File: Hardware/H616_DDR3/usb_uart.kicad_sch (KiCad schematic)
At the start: 5 parts, among them J3 USB_C_Receptacle_USB2.0

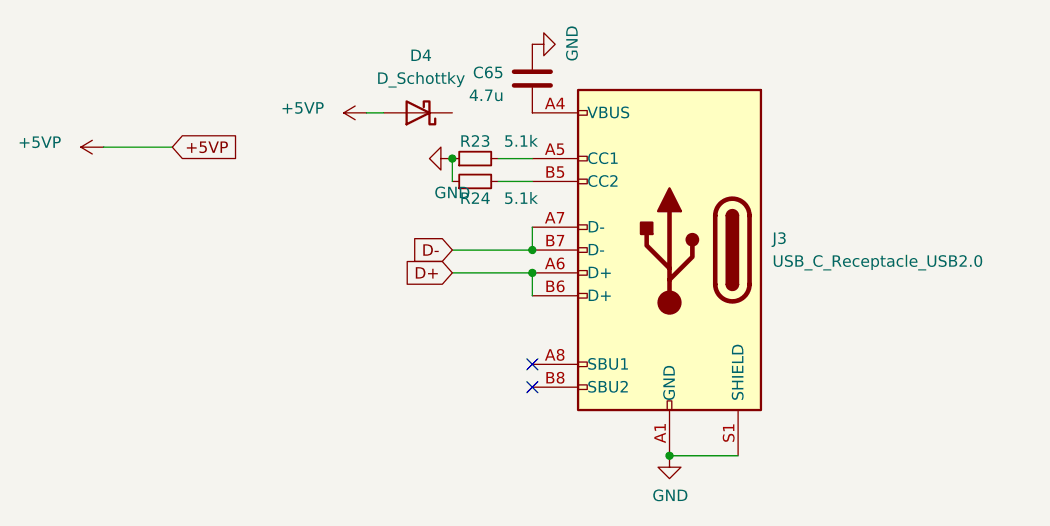
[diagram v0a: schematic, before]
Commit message: trace
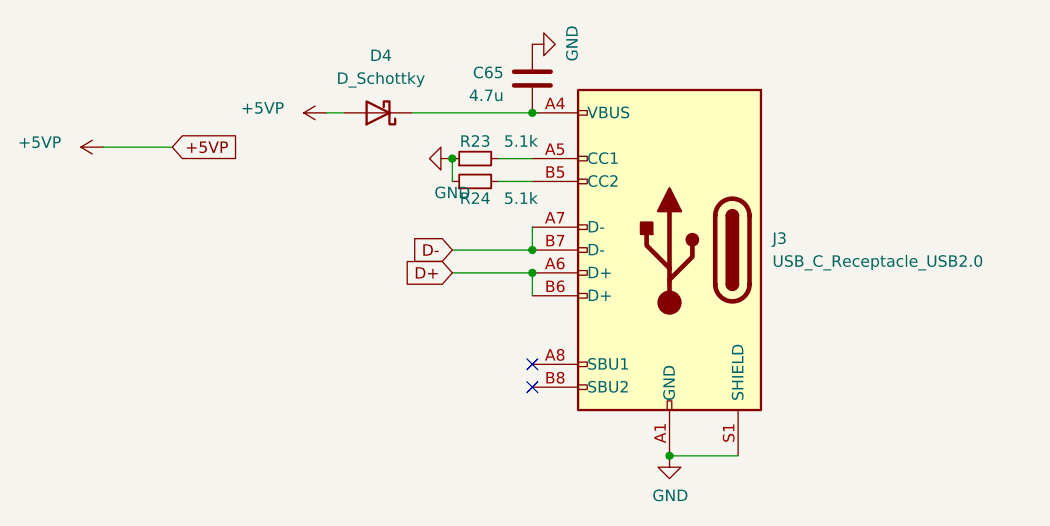
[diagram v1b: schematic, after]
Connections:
- net at C65.2, J3.A4 (VBUS), J3.A9 (VBUS)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: now also D4.1 (K)
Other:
- moved on the sheet: D4
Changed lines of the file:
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@@
+	)
+	(junction
+		(at 165.735 110.49)
+		(diameter 0)
+		(color 0 0 0 0)
 	)
 	(junction
@@
 	(wire
 		(pts
+			(xy 152.4 110.49) (xy 165.735 110.49)
+		)
+		(stroke
+			(width 0)
+			(type default)
+		)
+	)
+	(wire
+		(pts
 			(xy 156.845 115.57) (xy 156.845 118.11)
 		)
@@
 	(wire
 		(pts
-			(xy 147.32 110.49) (xy 149.225 110.49)
+			(xy 142.875 110.49) (xy 144.78 110.49)
 		)
 		(stroke
@@
 		(pts
 			(xy 165.735 123.19) (xy 165.735 125.73)
+		)
+		(stroke
+			(width 0)
+			(type default)
+		)
+	)
+	(wire
+		(pts
+			(xy 165.735 110.49) (xy 166.37 110.49)
 		)
 		(stroke
@@
 	(symbol
 		(lib_id "power:+5VP")
-		(at 147.32 110.49 90)
+		(at 142.875 110.49 90)
 		(unit 1)
 		(body_style 1)
@@
 		(dnp no)
 		(property "Reference" "#PWR089"
-			(at 151.13 110.49 0)
+			(at 146.685 110.49 0)
 			(hide yes)
 			(show_name no)
@@
 		)
 		(property "Value" "+5VP"
-			(at 137.795 109.982 90)
+			(at 133.35 109.982 90)
 			(show_name no)
 			(do_not_autoplace no)
@@
 		)
 		(property "Footprint" ""
-			(at 147.32 110.49 0)
+			(at 142.875 110.49 0)
 			(hide yes)
 			(show_name no)
@@
 		)
 		(property "Datasheet" ""
-			(at 147.32 110.49 0)
+			(at 142.875 110.49 0)
 			(hide yes)
 			(show_name no)
@@
 		)
 		(property "Description" ""
-			(at 147.32 110.49 0)
+			(at 142.875 110.49 0)
 			(hide yes)
 			(show_name no)
@@
 	(symbol
 		(lib_id "Device:D_Schottky")
-		(at 153.035 110.49 180)
+		(at 148.59 110.49 180)
 		(unit 1)
 		(body_style 1)
@@
 		(fields_autoplaced yes)
 		(property "Reference" "D4"
-			(at 153.3525 104.14 0)
+			(at 148.9075 104.14 0)
 			(show_name no)
 			(do_not_autoplace no)
@@
 		)
 		(property "Value" "D_Schottky"
-			(at 153.3525 106.68 0)
+			(at 148.9075 106.68 0)
 			(show_name no)
 			(do_not_autoplace no)
@@
 		)
 		(property "Footprint" "Diode_SMD:D_SOD-323_HandSoldering"
-			(at 153.035 110.49 0)
+			(at 148.59 110.49 0)
 			(hide yes)
 			(show_name no)
@@
 		)
 		(property "Datasheet" ""
-			(at 153.035 110.49 0)
+			(at 148.59 110.49 0)
 			(hide yes)
 			(show_name no)
@@
 		)
 		(property "Description" ""
-			(at 153.035 110.49 0)
-			(hide yes)
-			(show_name no)
+			(at 148.59 110.49 0)
+			(hide yes)
+			(show_name no)
